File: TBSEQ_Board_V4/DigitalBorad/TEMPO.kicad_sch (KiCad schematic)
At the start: 1 part, among them J1 Conn_01x05

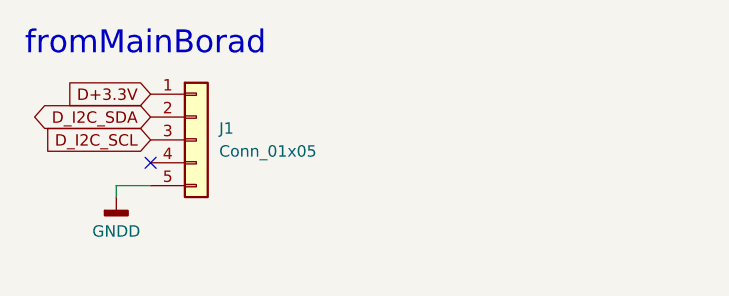
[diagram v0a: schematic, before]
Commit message: TBSEQ_BoardV4
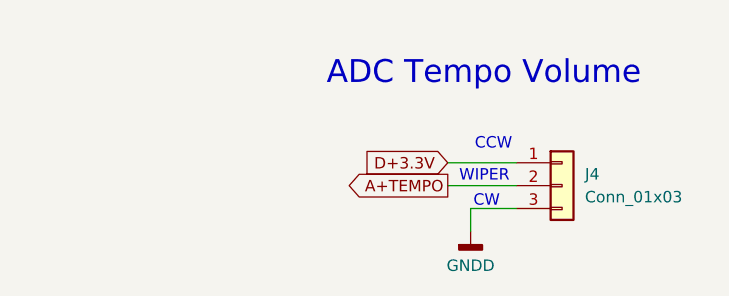
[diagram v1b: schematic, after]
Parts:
- removed J1: Conn_01x05, Connector_PinSocket_2.54mm:PinSocket_1x05_P2.54mm_Vertical, symbol Connector_Generic:Conn_01x05
- added J4: Conn_01x03, Connector_PinSocket_2.54mm:PinSocket_1x03_P2.54mm_Vertical, symbol Connector_Generic:Conn_01x03
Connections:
- net D+3.3V: now also J4.1 (Pin_1)
- net GNDD: now also J4.3 (Pin_3)
- new net A+TEMPO: J4.2 (Pin_2)
- no-connect marks 1 -> 0
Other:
- note added: "ADC Tempo Volume"
- note added: "CCW"
- note added: "CW"
- note added: "WIPER"
- note removed: "fromMainBorad"
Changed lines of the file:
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@@
 	(generator_version "9.0")
 	(paper "A4")
-	(text "fromMainBorad"
-		(exclude_from_sim no)
-		(at 64.77 38.862 0)
+	(text "CW"
+		(exclude_from_sim no)
+		(at 116.078 56.388 0)
+		(effects
+			(font
+				(size 1.27 1.27)
+			)
+		)
+	)
+	(text "WIPER"
+		(exclude_from_sim no)
+		(at 115.824 53.594 0)
+		(effects
+			(font
+				(size 1.27 1.27)
+			)
+		)
+	)
+	(text "ADC Tempo Volume"
+		(exclude_from_sim no)
+		(at 98.298 42.164 0)
 		(effects
 			(font
@@
 		)
 	)
-	(no_connect
-		(at 78.74 52.07)
-	)
-	(wire
-		(pts
-			(xy 78.74 54.61) (xy 74.93 54.61)
-		)
-		(stroke
-			(width 0)
-			(type default)
-		)
-	)
-	(wire
-		(pts
-			(xy 74.93 54.61) (xy 74.93 55.88)
-		)
-		(stroke
-			(width 0)
-			(type default)
-		)
-	)
-	(global_label "D_I2C_SDA"
-		(shape bidirectional)
-		(at 78.74 46.99 180)
-		(fields_autoplaced yes)
-		(effects
-			(font
-				(size 1.27 1.27)
-			)
-			(justify right)
-		)
-		(property "Intersheetrefs" "${INTERSHEET_REFS}"
-			(at 68.6186 46.99 0)
-			(effects
-				(font
-					(size 1.27 1.27)
-				)
-				(justify right)
-				(hide yes)
-			)
-		)
-	)
-	(global_label "D_I2C_SCL"
-		(shape input)
-		(at 78.74 49.53 180)
-		(fields_autoplaced yes)
-		(effects
-			(font
-				(size 1.27 1.27)
-			)
-			(justify right)
-		)
-		(property "Intersheetrefs" "${INTERSHEET_REFS}"
-			(at 68.6186 49.53 0)
-			(effects
-				(font
-					(size 1.27 1.27)
-				)
-				(justify right)
-				(hide yes)
-			)
+	(text "CCW"
+		(exclude_from_sim no)
+		(at 116.84 50.038 0)
+		(effects
+			(font
+				(size 1.27 1.27)
+			)
+		)
+	)
+	(wire
+		(pts
+			(xy 119.38 57.15) (xy 114.3 57.15)
+		)
+		(stroke
+			(width 0)
+			(type default)
+		)
+	)
+	(wire
+		(pts
+			(xy 111.76 54.61) (xy 119.38 54.61)
+		)
+		(stroke
+			(width 0)
+			(type default)
+		)
+	)
+	(wire
+		(pts
+			(xy 111.76 52.07) (xy 119.38 52.07)
+		)
+		(stroke
+			(width 0)
+			(type default)
+		)
+	)
+	(wire
+		(pts
+			(xy 114.3 57.15) (xy 114.3 59.69)
+		)
+		(stroke
+			(width 0)
+			(type default)
 		)
 	)
 	(global_label "D+3.3V"
 		(shape input)
-		(at 78.74 44.45 180)
+		(at 111.76 52.07 180)
 		(fields_autoplaced yes)
 		(effects
@@
 		)
 		(property "Intersheetrefs" "${INTERSHEET_REFS}"
-			(at 68.8 44.45 0)
+			(at 101.82 52.07 0)
 			(effects
 				(font
@@
 		)
 	)
+	(global_label "A+TEMPO"
+		(shape output)
+		(at 111.76 54.61 180)
+		(fields_autoplaced yes)
+		(effects
+			(font
+				(size 1.27 1.27)
+			)
+			(justify right)
+		)
+		(property "Intersheetrefs" "${INTERSHEET_REFS}"
+			(at 99.9453 54.61 0)
+			(effects
+				(font
+					(size 1.27 1.27)
+				)
+				(justify right)
+				(hide yes)
+			)
+		)
+	)
 	(symbol
-		(lib_id "Connector_Generic:Conn_01x05")
-		(at 83.82 49.53 0)
+		(lib_id "power:GNDD")
+		(at 114.3 59.69 0)
+		(unit 1)
+		(exclude_from_sim no)
+		(in_bom yes)
+		(on_board yes)
+		(dnp no)
+		(property "Reference" "#PWR045"
+			(at 114.3 66.04 0)
+			(effects
+				(font
+					(size 1.27 1.27)
+				)
+				(hide yes)
+			)
+		)
+		(property "Value" "GNDD"
+			(at 114.3 63.5 0)
+			(effects
+				(font
+					(size 1.27 1.27)
+				)
+			)
+		)
+		(property "Footprint" ""
+			(at 114.3 59.69 0)
+			(effects
+				(font
+					(size 1.27 1.27)
+				)
+				(hide yes)
+			)
+		)
+		(property "Datasheet" ""
+			(at 114.3 59.69 0)
+			(effects
+				(font
+					(size 1.27 1.27)
+				)
+				(hide yes)
+			)
+		)
+		(property "Description" "Power symbol creates a global label with name \"GNDD\" , digital ground"
+			(at 114.3 59.69 0)
+			(effects
+				(font
+					(size 1.27 1.27)
+				)
+				(hide yes)
+			)
+		)
+		(pin "1"
+		)
+		(instances
+			(project "mainBorad_R1"
+				(path "/83af791a-9776-40a7-82ad-9528ff7474b8/67c88aa0-cd33-4e9c-b3f5-33809b562701"
+					(reference "#PWR045")
+					(unit 1)
+				)
+			)
+		)
+	)
+	(symbol
+		(lib_id "Connector_Generic:Conn_01x03")
+		(at 124.46 54.61 0)
 		(unit 1)
 		(exclude_from_sim no)
@@
 		(dnp no)
 		(fields_autoplaced yes)
-		(property "Reference" "J1"
-			(at 86.36 48.2599 0)
+		(property "Reference" "J4"
+			(at 127 53.3399 0)
 			(effects
 				(font
@@
 			)
 		)
-		(property "Value" "Conn_01x05"
-			(at 86.36 50.7999 0)
+		(property "Value" "Conn_01x03"
+			(at 127 55.8799 0)
 			(effects
 				(font
@@
 			)
 		)
-		(property "Footprint" "Connector_PinSocket_2.54mm:PinSocket_1x05_P2.54mm_Vertical"
-			(at 83.82 49.53 0)
+		(property "Footprint" "Connector_PinSocket_2.54mm:PinSocket_1x03_P2.54mm_Vertical"
+			(at 124.46 54.61 0)
 			(effects
 				(font
@@
 		)
 		(property "Datasheet" "~"
-			(at 83.82 49.53 0)
-			(effects
-				(font
-					(size 1.27 1.27)
-				)
-				(hide yes)
-			)
-		)
-		(property "Description" "Generic connector, single row, 01x05, script generated (kicad-library-utils/schlib/autogen/connector/)"
-			(at 83.82 49.53 0)
-			(effects
-				(font
-					(size 1.27 1.27)
-				)
-				(hide yes)
-			)
-		)
-		(property "Sim.Library" ""
-			(at 83.82 49.53 0)
-			(effects
-				(font
-					(size 1.27 1.27)
-				)
-				(hide yes)
-			)
-		)
-		(property "Sim.Name" ""
-			(at 83.82 49.53 0)
-			(effects
-				(font
-					(size 1.27 1.27)
-				)
-				(hide yes)
-			)
+			(at 124.46 54.61 0)
+			(effects
+				(font
+					(size 1.27 1.27)
+				)
+				(hide yes)
+			)
+		)
+		(property "Description" "Generic connector, single row, 01x03, script generated (kicad-library-utils/schlib/autogen/connector/)"
+			(at 124.46 54.61 0)
+			(effects
+				(font
+					(size 1.27 1.27)
+				)
+				(hide yes)
+			)
+		)
+		(pin "2"
 		)
 		(pin "1"
 		)
-		(pin "2"
-		)
-		(pin "4"
-		)
-		(pin "5"
-		)
 		(pin "3"
 		)
 		(instances
-			(project "panelBoard"
-				(path "/e4888aad-78d5-4afc-b382-d3fab1889a4d/1a1a0aa4-57dd-497b-b0ec-216c90fc74ae"
-					(reference "J1")
+			(project ""
+				(path "/83af791a-9776-40a7-82ad-9528ff7474b8/67c88aa0-cd33-4e9c-b3f5-33809b562701"
+					(reference "J4")
 					(unit 1)
 				)
-			)
-		)
-	)
-	(symbol
-		(lib_id "power:GNDD")
-		(at 74.93 55.88 0)
-		(unit 1)
-		(exclude_from_sim no)
-		(in_bom yes)
-		(on_board yes)
-		(dnp no)
-		(fields_autoplaced yes)
-		(property "Reference" "#PWR03"
-			(at 74.93 62.23 0)
-			(effects
-				(font
-					(size 1.27 1.27)
-				)
-				(hide yes)
-			)
-		)
-		(property "Value" "GNDD"
-			(at 74.93 59.69 0)
-			(effects
-				(font
-					(size 1.27 1.27)
-				)
-			)
-		)
-		(property "Footprint" ""
-			(at 74.93 55.88 0)
-			(effects
-				(font
-					(size 1.27 1.27)
-				)
-				(hide yes)
-			)
-		)
-		(property "Datasheet" ""
-			(at 74.93 55.88 0)
-			(effects
-				(font
-					(size 1.27 1.27)
-				)
-				(hide yes)
-			)
-		)
-		(property "Description" "Power symbol creates a global label with name \"GNDD\" , digital ground"
-			(at 74.93 55.88 0)
-			(effects
-				(font
-					(size 1.27 1.27)
-				)
-				(hide yes)
-			)
-		)
-		(pin "1"
-		)
-		(instances
-			(project "panelBoard"
-				(path "/e4888aad-78d5-4afc-b382-d3fab1889a4d/1a1a0aa4-57dd-497b-b0ec-216c90fc74ae"
-					(reference "#PWR03")
-					(unit 1)
-				)
